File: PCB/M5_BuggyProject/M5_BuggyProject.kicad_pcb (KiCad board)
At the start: 2 copper layers, 40.6 x 74.9 mm, 18 parts, among them J1 XT60

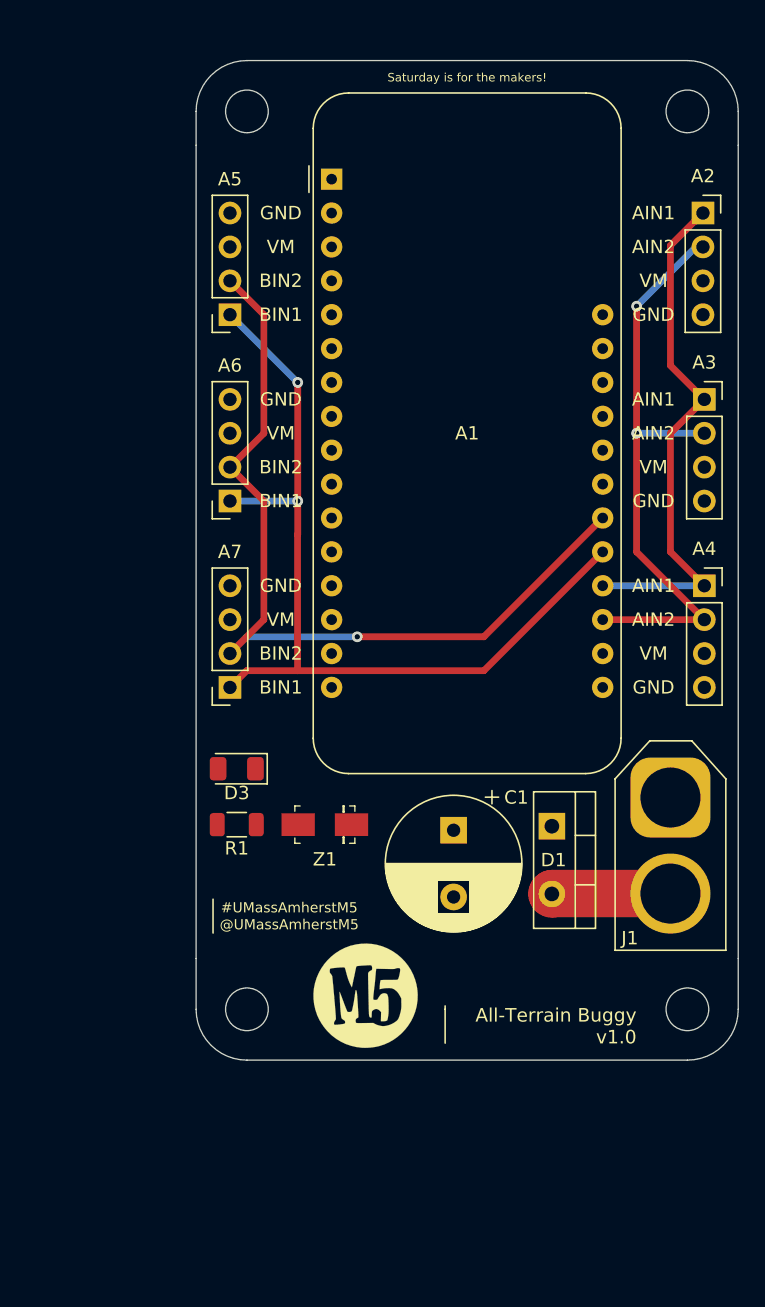
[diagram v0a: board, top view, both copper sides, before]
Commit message: Finalised PCB for v1.0
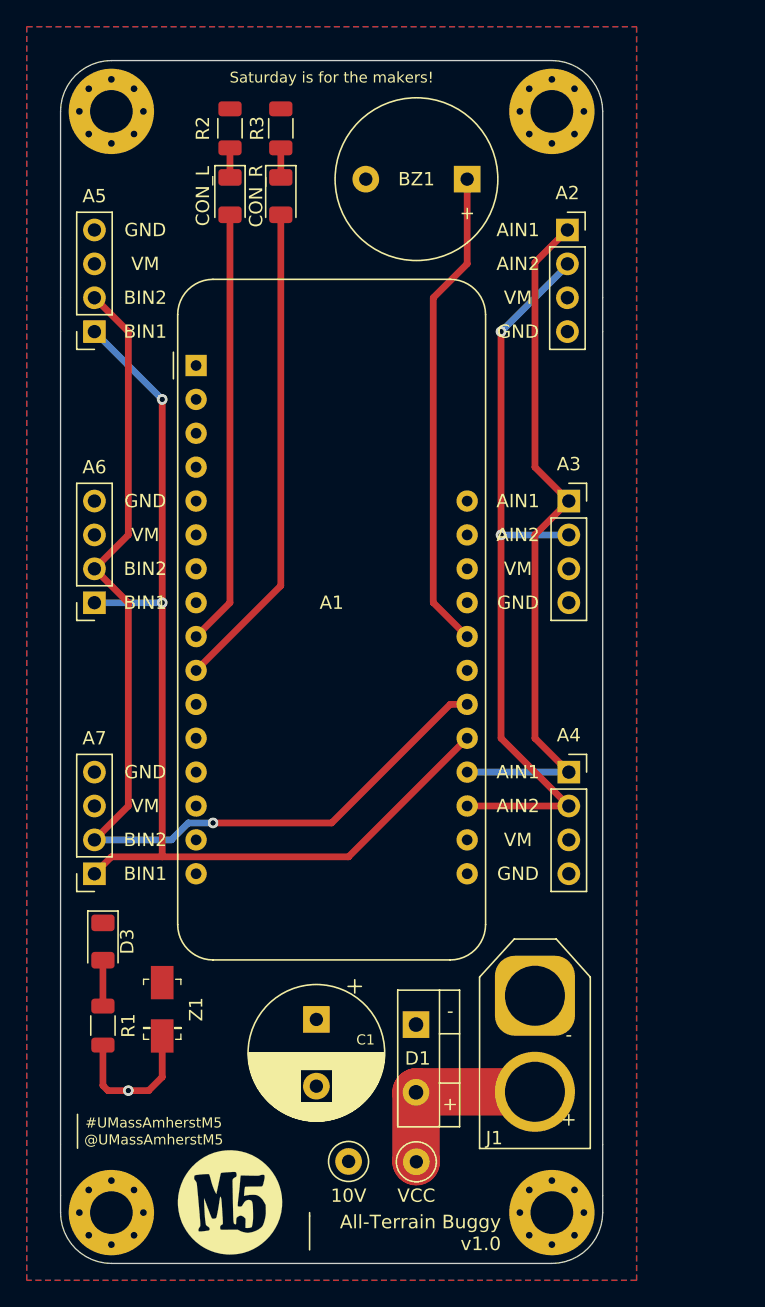
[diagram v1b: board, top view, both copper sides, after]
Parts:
- removed REF** (x4): MountingHole_3.2mm_M3, MountingHole:MountingHole_3.2mm_M3
- added BZ1: BEEP, Buzzer_Beeper:Buzzer_12x9.5RM7.6, F.Cu at (107.2, 44.2)
- added D2: ORANGE, LED_SMD:LED_1206_3216Metric, F.Cu at (89.4, 45.5)
- added D4: ORANGE, LED_SMD:LED_1206_3216Metric, F.Cu at (93.2, 45.5)
- added H1: M, MountingHole:MountingHole_3.2mm_M3_Pad_Via, F.Cu at (80.5, 39.1)
- added H2: M, MountingHole:MountingHole_3.2mm_M3_Pad_Via, F.Cu at (113.5, 39.1)
- added H3: M, MountingHole:MountingHole_3.2mm_M3_Pad_Via, F.Cu at (113.5, 121.7)
- added H4: M, MountingHole:MountingHole_3.2mm_M3_Pad_Via, F.Cu at (80.5, 121.7)
- added J2: VCC, TestPoint:TestPoint_Loop_D1.80mm_Drill1.0mm_Beaded, F.Cu at (103.4, 117.9)
- added J3: 10V, TestPoint:TestPoint_Loop_D1.80mm_Drill1.0mm_Beaded, F.Cu at (98.3, 117.8)
- added R2: 100, Resistor_SMD:R_1206_3216Metric, F.Cu at (89.4, 40.4)
- added R3: 100, Resistor_SMD:R_1206_3216Metric, F.Cu at (93.2, 40.4)
- D3: value LED -> BLUE
- R1: value 698 -> 330
- moved G*** 18.5 mm to (89.4, 120.9)
- moved Z1 18.4 mm to (84.3, 106.4), turned to 90 degrees
- moved R1 18.1 mm to (79.9, 107.6), turned to 270 degrees
- moved D1 18.0 mm to (103.4, 107.6)
- moved J1 18.0 mm to (112.3, 105.4)
- moved C1 17.5 mm to (95.9, 107.2)
- moved A1 17.3 mm to (86.9, 58.2)
- moved A4 17.3 mm to (114.8, 88.6)
- moved A7 17.3 mm to (79.2, 96.3)
- moved D3 16.4 mm to (79.9, 101.3), turned to 270 degrees
- moved A6 12.7 mm to (79.2, 75.9)
- moved A3 12.7 mm to (114.8, 68.3)
- moved A2 10.2 mm to (114.7, 48.0)
- moved A5 10.2 mm to (79.2, 55.6)
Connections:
- net +12V renamed +10V
- net Net-(A1-Pad8) renamed CHANNEL_3
- A1 pad 10: Net-(A1-Pad10) -> CONFIG_R
- A1 pad 24: Net-(A1-Pad24) -> BEEP
- A1 pad 9: Net-(A1-Pad9) -> CONFIG_L
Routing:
- net CONFIG_R: track 0.00 -> 36.8 mm
- net BEEP: track 0.00 -> 36.4 mm
- net CONFIG_L: track 0.00 -> 32.7 mm
- net BIN2: track 64.3 -> 77.0 mm
- net AIN1: track 39.7 -> 52.4 mm
- net BIN1: track 66.0 -> 78.7 mm
- net AIN2: track 45.1 -> 57.5 mm
- net +10V: track 0.00 -> 11.1 mm, vias 0 -> 1
- net VCC: track 8.90 -> 14.1 mm
- net Net-(D3-Pad2): track 0.00 -> 3.44 mm
- net Net-(D4-Pad1): track 0.00 -> 2.22 mm
- net Net-(D2-Pad1): track 0.00 -> 2.22 mm
- added copper zone on B.Cu, net +10V
- added copper zone on F.Cu, net GND
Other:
- board size 40.6 x 74.9 mm -> 40.6 x 90.2 mm
- board text added: "+"
- board text added: "-"
- board text added: "10V"
- board text added: "CON_L"
- board text added: "CON_R"
- board text added: "Designers: Akshat Sahay 2023, Sebastian Armstrong 2024 License: CC BY 4.0"
- board text added: "VCC"
